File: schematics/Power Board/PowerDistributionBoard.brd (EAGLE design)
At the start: 66 x 53.3 mm, 11 parts

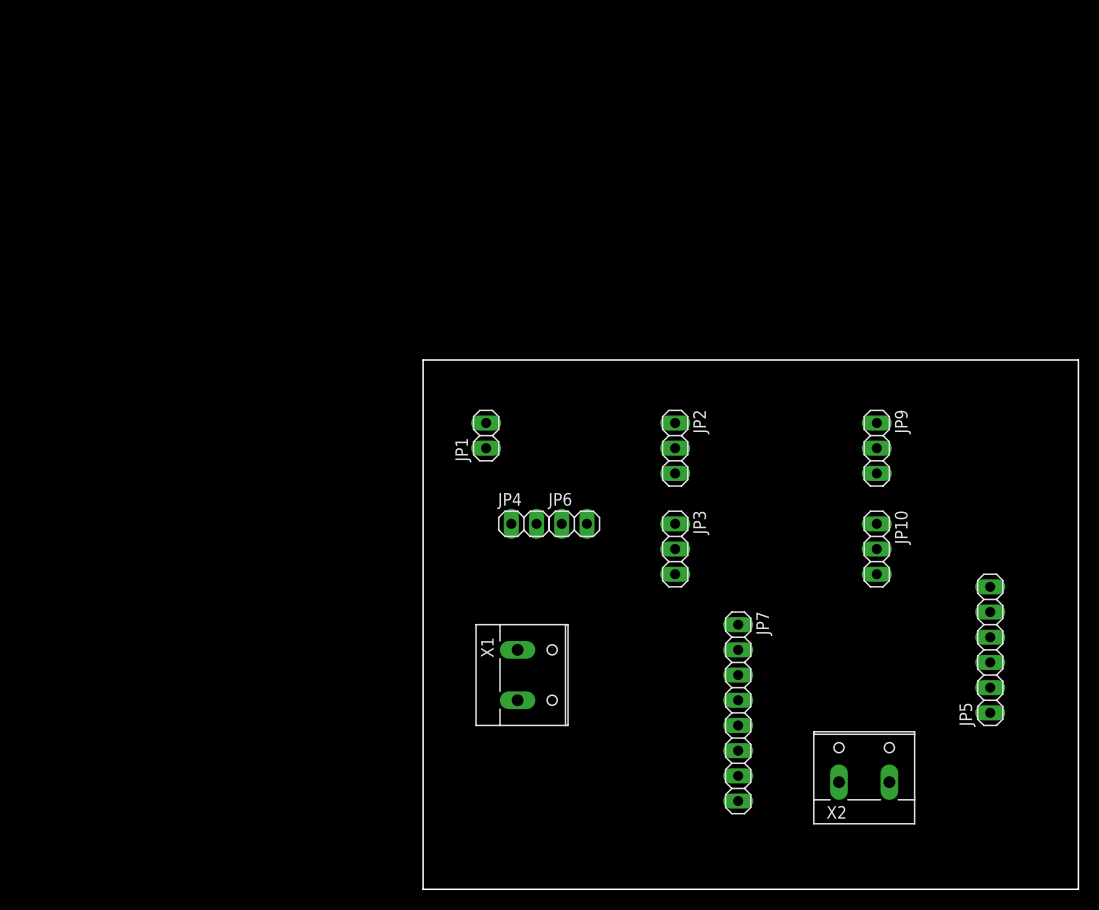
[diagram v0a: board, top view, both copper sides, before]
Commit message: Updated Most Recent PCB's
Changed both directories with the most up to date schematics.
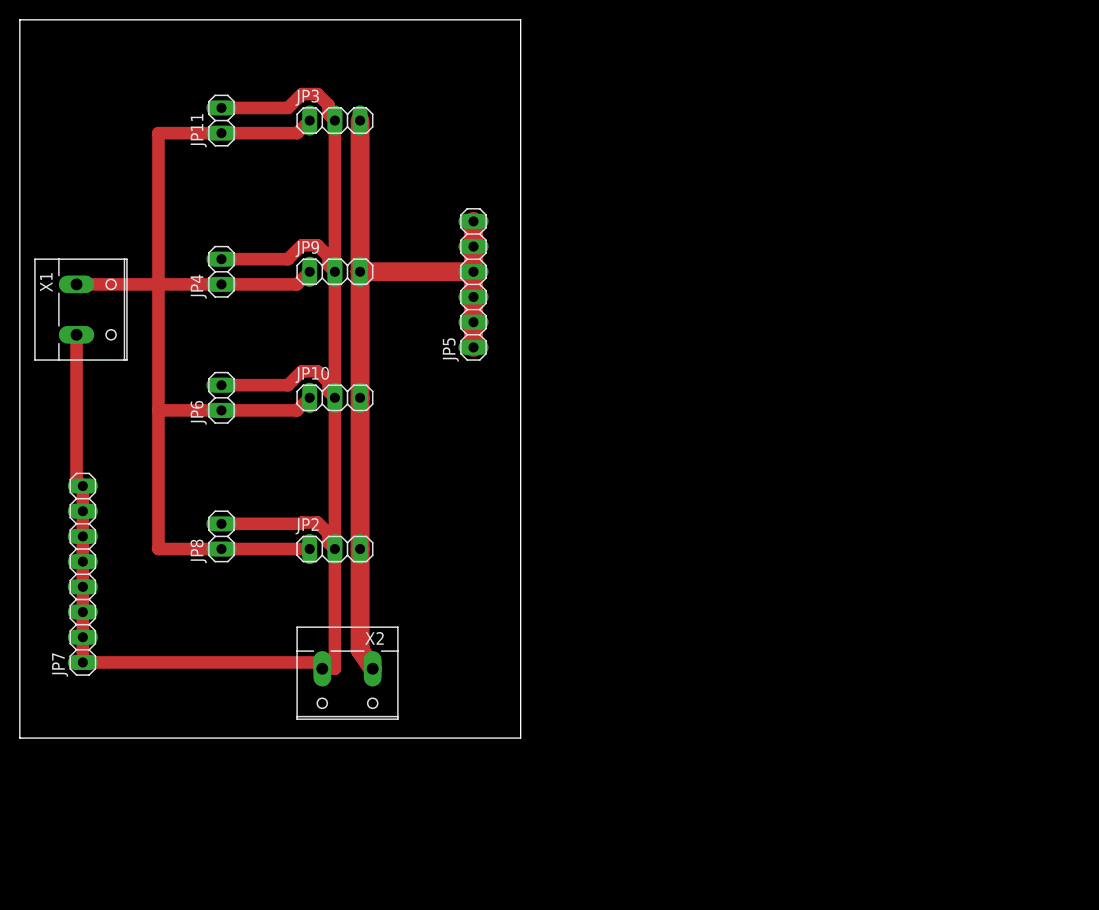
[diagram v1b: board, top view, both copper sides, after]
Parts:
- removed JP1: (no value), pinhead:1X02
- added JP11, JP8: (no value), pinhead:1X02
- moved JP7 67.5 mm to (6.35, 22.9), turned to 90 degrees
- moved JP5 63.8 mm to (45.7, 52.1)
- moved X1 57.7 mm to (6.35, 49.5)
- moved JP9 57.4 mm to (31.8, 53.3), turned to 0 degrees
- moved JP10 56.7 mm to (31.8, 40.6), turned to 0 degrees
- moved JP3 55.1 mm to (31.8, 68.6), turned to 0 degrees
- moved X2 53.1 mm to (33.0, 12.7), turned to 180 degrees
- moved JP4 39.7 mm to (20.3, 53.3), turned to 90 degrees
- moved JP6 37.8 mm to (20.3, 40.6), turned to 90 degrees
- moved JP2 35.8 mm to (31.8, 25.4), turned to 0 degrees
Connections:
- removed net N$2: JP4.2, JP6.1
- removed net V-IN: JP10.1, JP2.1, JP3.1, JP6.2, JP9.1
- net COMMON-GND: now also JP11.2, JP4.2, JP6.2, JP8.2
- net N$1: now also JP10.1, JP11.1, JP2.1, JP3.1, JP6.1, JP8.1, JP9.1; no longer JP1.1, JP1.2
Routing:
- net COMMON-GND: track 0.00 -> 168.6 mm
- net N$1: track 0.00 -> 112.7 mm
- net SENSOR-5V+: track 0.00 -> 79.8 mm
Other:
- board size 66 x 53.3 mm -> 50.5 x 72.4 mm
